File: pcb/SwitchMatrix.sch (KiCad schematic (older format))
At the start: 112 parts, among them K0 KEYSW, K1 KEYSW, K10 KEYSW, K11 KEYSW, K12 KEYSW, K13 KEYSW, K14 KEYSW, K15 KEYSW, K2 KEYSW, K20 KEYSW, K21 KEYSW, K22 KEYSW, K23 KEYSW, K24 KEYSW, K25 KEYSW, K26 KEYSW, K27 KEYSW, K3 KEYSW, K30 KEYSW, K31 KEYSW, K32 KEYSW, K33 KEYSW, K34 KEYSW, K35 KEYSW, K36 KEYSW, K37 KEYSW, K4 KEYSW, K42 KEYSW, K43 KEYSW, K44 KEYSW, K45 KEYSW, K46 KEYSW, K47 KEYSW, K5 KEYSW, K52 KEYSW, K53 KEYSW, K54 KEYSW, K55 KEYSW, K56 KEYSW, K57 KEYSW, K60 KEYSW, K61 KEYSW, K62 KEYSW, K63 KEYSW, K64 KEYSW, K65 KEYSW, K66 KEYSW, K67 KEYSW, K70 KEYSW, K71 KEYSW, K72 KEYSW, K73 KEYSW, K74 KEYSW, K75 KEYSW, K76 KEYSW, K77 KEYSW

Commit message: Most pcb of layout done
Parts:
- D00: renamed from D0; footprint Keyboard_Parts:D_axial -> Diode_SMD:D_1806_4516Metric_Pad1.57x1.80mm_HandSolder
- D01: renamed from D1; footprint Keyboard_Parts:D_axial -> Diode_SMD:D_1806_4516Metric_Pad1.57x1.80mm_HandSolder
- D02: renamed from D2; footprint Keyboard_Parts:D_axial -> Diode_SMD:D_1806_4516Metric_Pad1.57x1.80mm_HandSolder
- D03: renamed from D3; footprint Keyboard_Parts:D_axial -> Diode_SMD:D_1806_4516Metric_Pad1.57x1.80mm_HandSolder
- D04: renamed from D4; footprint Keyboard_Parts:D_axial -> Diode_SMD:D_1806_4516Metric_Pad1.57x1.80mm_HandSolder
- D05: renamed from D5; footprint Keyboard_Parts:D_axial -> Diode_SMD:D_1806_4516Metric_Pad1.57x1.80mm_HandSolder
- D10, D11, D12, D13, D14, D15, D20, D21, D22, D23, D24, D25, D26, D27, D30, D31, D32, D33, D34, D35, D36, D37, D42, D43, D44, D45, D46, D47, D52, D53, D54, D55, D56, D57, D60, D61, D62, D63, D64, D65, D66, D67, D70, D71, D72, D73, D74, D75, D76, D77: footprint Keyboard_Parts:D_axial -> Diode_SMD:D_1806_4516Metric_Pad1.57x1.80mm_HandSolder
- K00: renamed from K0; footprint keyswitches:Kailh_socket_vias -> keyswitches:Kailh_socket_via_on_pin_one
- K01: renamed from K1; footprint keyswitches:Kailh_socket_vias -> keyswitches:Kailh_socket_via_on_pin_one
- K02: renamed from K2; footprint keyswitches:Kailh_socket_vias -> keyswitches:Kailh_socket_via_on_pin_one
- K03: renamed from K3; footprint keyswitches:Kailh_socket_vias -> keyswitches:Kailh_socket_via_on_pin_one
- K04: renamed from K4; footprint keyswitches:Kailh_socket_vias -> keyswitches:Kailh_socket_via_on_pin_one
- K05: renamed from K5; footprint keyswitches:Kailh_socket_vias -> keyswitches:Kailh_socket_via_on_pin_one
- K10, K11, K12, K13, K14, K15, K20, K21, K22, K23, K24, K25, K26, K27, K30, K31, K32, K33, K34, K35, K36, K37, K42, K43, K44, K45, K46, K47, K52, K53, K54, K55, K56, K57, K60, K61, K62, K63, K64, K65, K66, K67, K70, K71, K72, K73, K74, K75, K76, K77: footprint keyswitches:Kailh_socket_vias -> keyswitches:Kailh_socket_via_on_pin_one
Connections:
- wire segments 284 -> 280

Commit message: Moved custom symbols & footprints into git submodules
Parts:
- K00, K01, K02, K03, K04, K05, K10, K11, K12, K13, K14, K15, K20, K21, K22, K23, K24, K25, K26, K27, K30, K31, K32, K33, K34, K35, K36, K37, K42, K43, K44, K45, K46, K47, K52, K53, K54, K55, K56, K57, K60, K61, K62, K63, K64, K65, K66, K67, K70, K71, K72, K73, K74, K75, K76, K77: footprint keyswitches:Kailh_socket_via_on_pin_one -> SVastaCustomParts:Kailh_socket_via_on_pin_one

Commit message: More layout work
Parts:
- D00, D01, D02, D03, D04, D05, D10, D11, D12, D13, D14, D15, D20, D21, D22, D23, D24, D25, D26, D27, D30, D31, D32, D33, D34, D35, D36, D37, D42, D43, D44, D45, D46, D47, D52, D53, D54, D55, D56, D57, D60, D61, D62, D63, D64, D65, D66, D67, D70, D71, D72, D73, D74, D75, D76, D77: footprint Diode_SMD:D_1806_4516Metric_Pad1.57x1.80mm_HandSolder -> SVastaCustomParts:D_MiniMELF_Handsoldering_Shorter_Pads

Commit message: Minor changes and started trackball module
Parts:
- removed D42, D43, D44, D45, D46, D47, D52, D53, D54, D55, D56, D57, D60, D61, D62, D63, D64, D65, D66, D67, D70, D71, D72, D73, D74, D75, D76, D77: D, SVastaCustomParts:D_MiniMELF_Handsoldering_Shorter_Pads, symbol Keyboard_Parts:D
- removed K42, K43, K44, K45, K46, K47, K52, K53, K54, K55, K56, K57, K60, K61, K62, K63, K64, K65, K66, K67, K70, K71, K72, K73, K74, K75, K76, K77: KEYSW, SVastaCustomParts:Kailh_socket_via_on_pin_one, symbol Keyboard_Parts:KEYSW
- D00, D01, D02, D03, D04, D05, D10, D11, D12, D13, D14, D15, D20, D21, D22, D23, D24, D25, D26, D27, D30, D31, D32, D33, D34, D35, D36, D37: footprint SVastaCustomParts:D_MiniMELF_Handsoldering_Shorter_Pads -> SVastaCustomParts:D_MiniMELF_Handsoldering_Shorter_Pads_DoubleSided; symbol Keyboard_Parts:D -> Keeb-rescue:D-Keyboard_Parts-Keeb-rescue
- K00, K01, K02, K03, K04, K05, K10, K11, K12, K13, K14, K15, K20, K21, K22, K23, K24, K25, K26, K27, K30, K31, K32, K33, K34, K35, K36, K37: footprint SVastaCustomParts:Kailh_socket_via_on_pin_one -> SVastaCustomParts:Kailh_socket_reversible; symbol Keyboard_Parts:KEYSW -> Keeb-rescue:KEYSW-Keyboard_Parts-Keeb-rescue
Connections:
- net labels removed: Row4, Row5, Row6, Row7
- wire segments 280 -> 140
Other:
- note removed: "Right Hand"

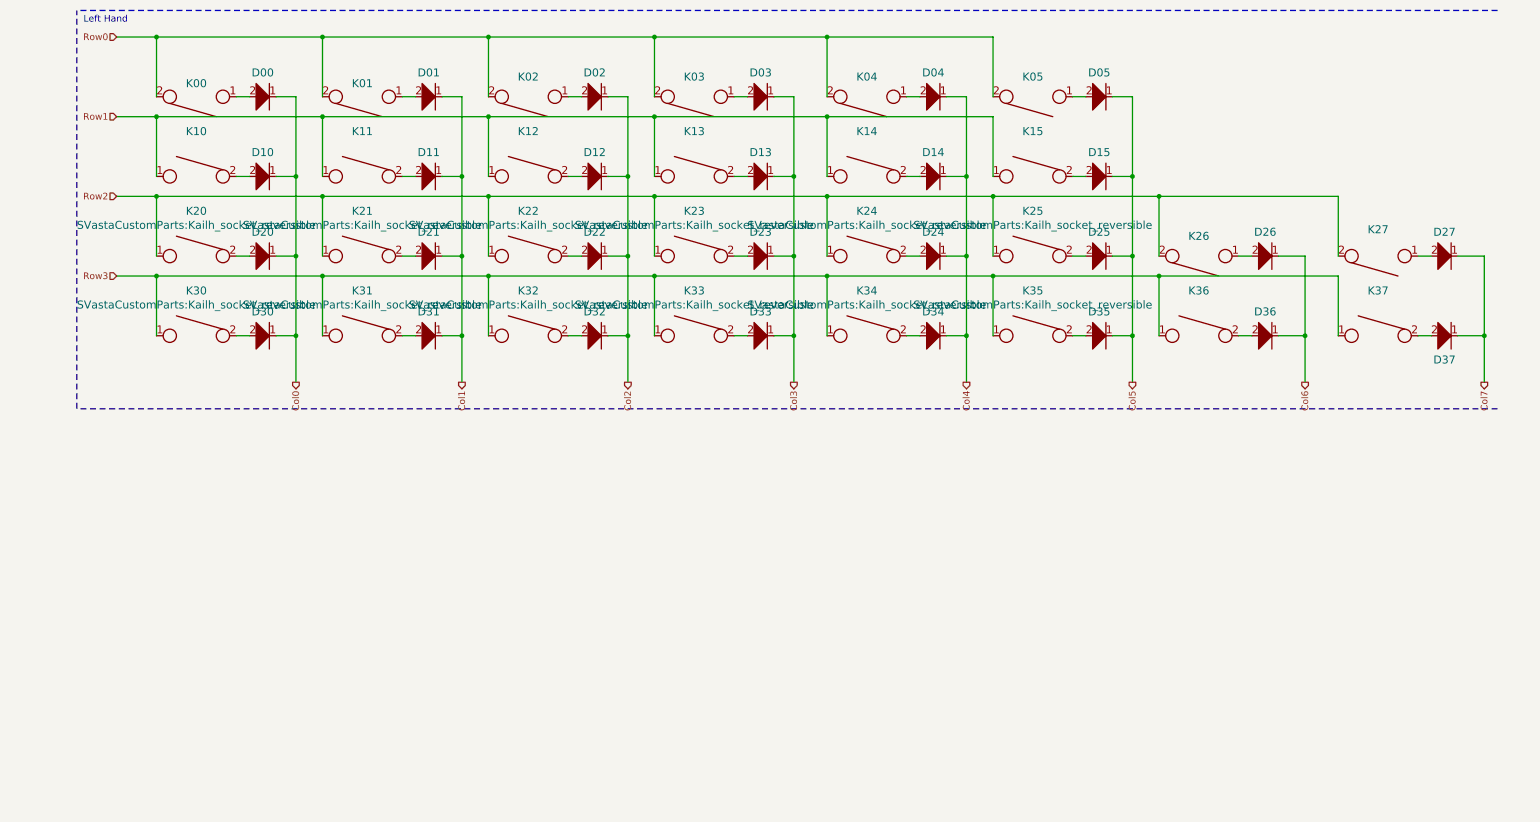
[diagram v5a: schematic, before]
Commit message: Fixed issues from test branch
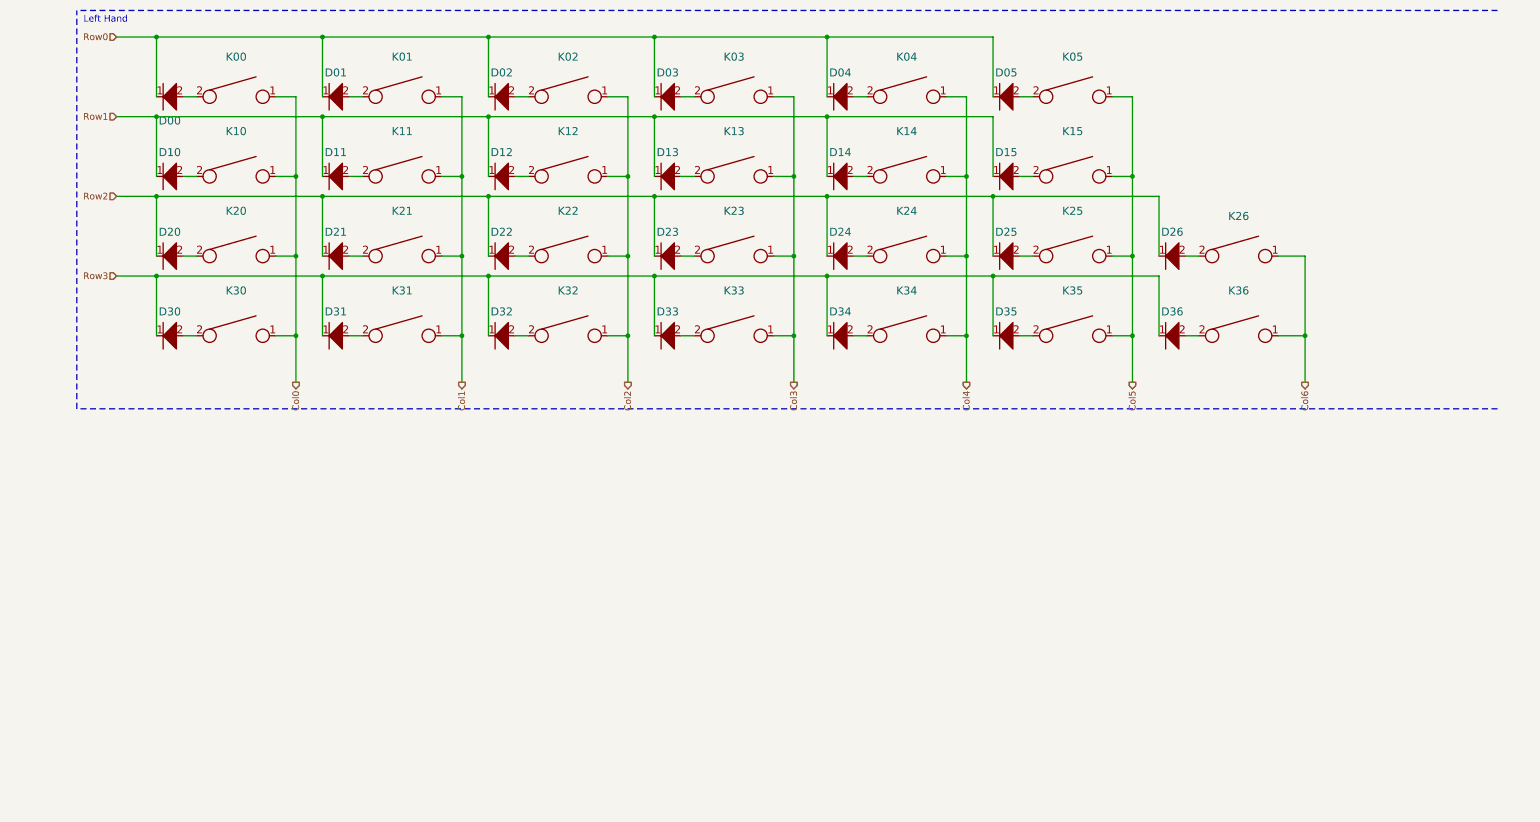
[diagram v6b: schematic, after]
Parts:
- removed D27, D37: D, SVastaCustomParts:D_MiniMELF_Handsoldering_Shorter_Pads_DoubleSided, symbol Keeb-rescue:D-Keyboard_Parts-Keeb-rescue
- removed K27, K37: KEYSW, SVastaCustomParts:Kailh_socket_reversible, symbol Keeb-rescue:KEYSW-Keyboard_Parts-Keeb-rescue
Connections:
- net Col0: now also K00.1, K10.1, K20.1, K30.1; no longer D00.1, D10.1, D20.1, D30.1
- net Col1: now also K01.1, K11.1, K21.1, K31.1; no longer D01.1, D11.1, D21.1, D31.1
- net Col2: now also K02.1, K12.1, K22.1, K32.1; no longer D02.1, D12.1, D22.1, D32.1
- net Col3: now also K03.1, K13.1, K23.1, K33.1; no longer D03.1, D13.1, D23.1, D33.1
- net Col4: now also K04.1, K14.1, K24.1, K34.1; no longer D04.1, D14.1, D24.1, D34.1
- net Col5: now also K05.1, K15.1, K25.1, K35.1; no longer D05.1, D15.1, D25.1, D35.1
- net Col6: now also K26.1, K36.1; no longer D26.1, D36.1
- net Row0: now also D00.1, D01.1, D02.1, D03.1, D04.1, D05.1; no longer K00.2, K01.2, K02.2, K03.2, K04.2, K05.2
- net Row1: now also D10.1, D11.1, D12.1, D13.1, D14.1, D15.1; no longer K10.1, K11.1, K12.1, K13.1, K14.1, K15.1
- net Row2: now also D20.1, D21.1, D22.1, D23.1, D24.1, D25.1, D26.1; no longer K20.1, K21.1, K22.1, K23.1, K24.1, K25.1, K26.2
- net Row3: now also D30.1, D31.1, D32.1, D33.1, D34.1, D35.1, D36.1; no longer K30.1, K31.1, K32.1, K33.1, K34.1, K35.1, K36.1
- net at D00.2: now also K00.2; no longer K00.1
- net at D01.2: now also K01.2; no longer K01.1
- net at D02.2: now also K02.2; no longer K02.1
- net at D03.2: now also K03.2; no longer K03.1
- net at D04.2: now also K04.2; no longer K04.1
- net at D05.2: now also K05.2; no longer K05.1
- net at D26.2: now also K26.2; no longer K26.1
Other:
- moved on the sheet: D00, D01, D02, D03, D04, D05, D10, D11, D12, D13, D14, D15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

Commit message: restarted layout
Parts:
- K26, K36: footprint SVastaCustomParts:Kailh_socket_reversible -> SVastaCustomParts:switch_off_board
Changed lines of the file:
@@
 F 0 "K26" H 9250 2650 60  0000 C CNN
 F 1 "KEYSW" H 9250 2250 60  0001 C CNN
-F 2 "SVastaCustomParts:Kailh_socket_reversible" H 9250 2583 60  0001 C CNN
+F 2 "SVastaCustomParts:switch_off_board" H 9250 2583 60  0001 C CNN
 F 3 "" H 9250 2350 60  0000 C CNN
 	1    9250 2350
@@
 F 0 "K36" H 9250 3289 60  0000 C CNN
 F 1 "KEYSW" H 9250 2850 60  0001 C CNN
-F 2 "SVastaCustomParts:Kailh_socket_reversible" H 9250 3183 60  0001 C CNN
+F 2 "SVastaCustomParts:switch_off_board" H 9250 3183 60  0001 C CNN
 F 3 "" H 9250 2950 60  0000 C CNN
 	1    9250 2950
